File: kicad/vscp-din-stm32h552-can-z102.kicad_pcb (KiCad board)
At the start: 2 copper layers, 47.8 x 84.8 mm, 39 parts, among them J1 Conn_01x05, J2 Conn_01x02, J3 Conn_01x06, J4 Conn_01x04, J5 Conn_01x04, J6 Conn_01x03, J7 Conn_01x05, J8 Conn_01x02, J9 Conn_01x02, U1 ESP32-C3-WROOM-02-N4, U2 LM2575-3.3BT, U3 SN65HVD232, U4 R-78B3.3-1.0 (Recom)

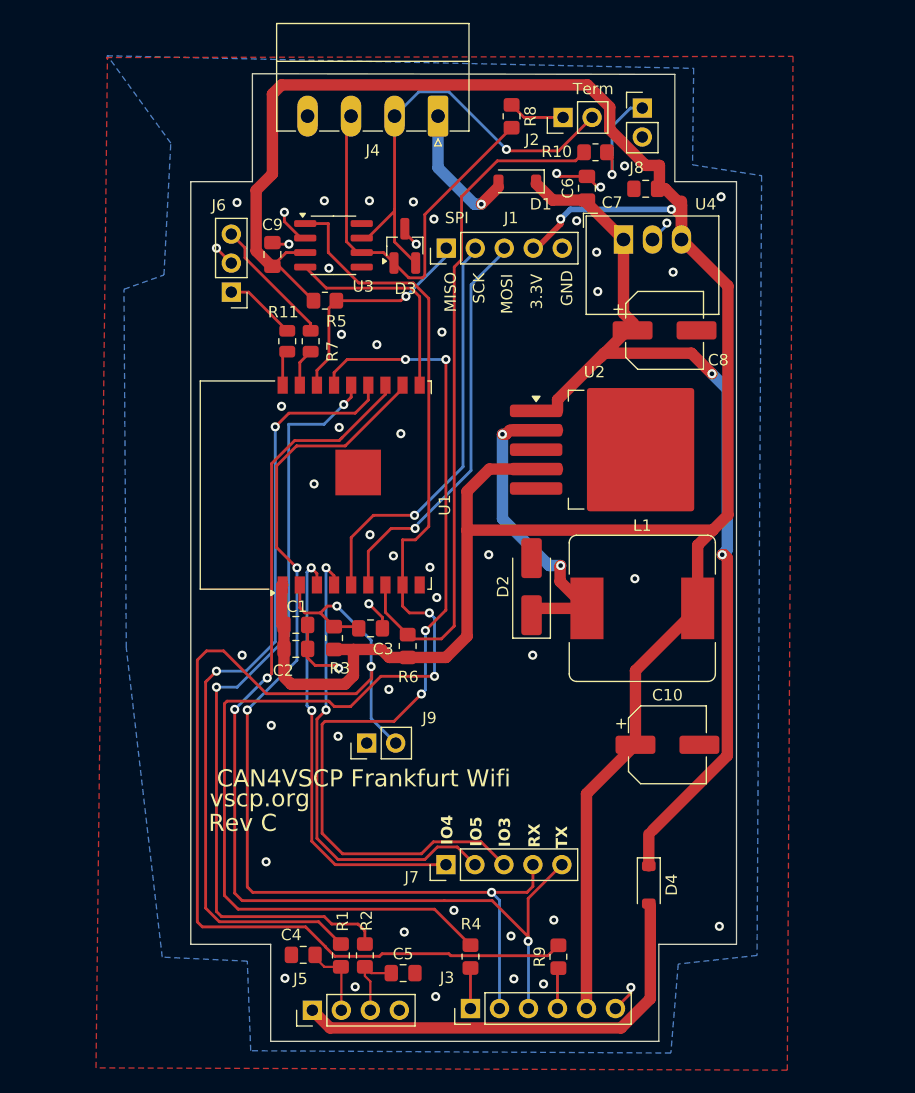
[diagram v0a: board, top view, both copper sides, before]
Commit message: Reversion A schema and PCB
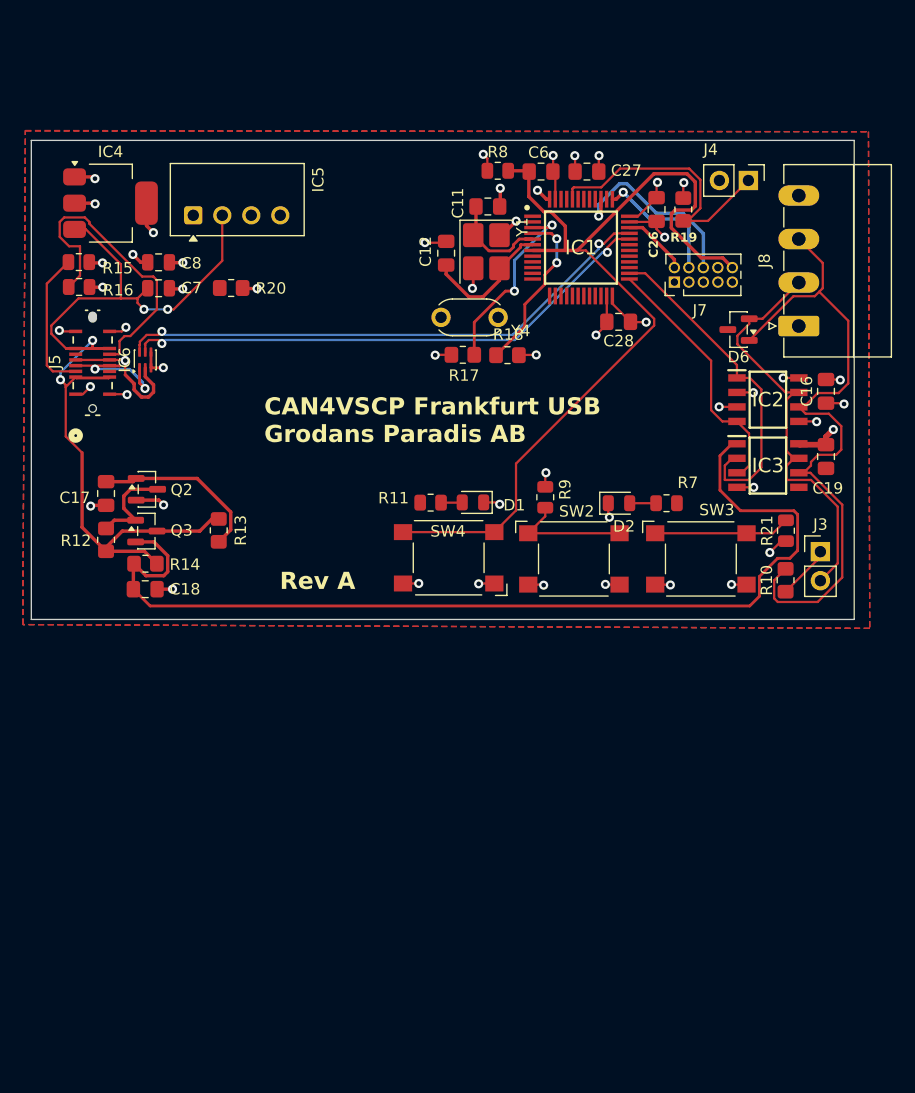
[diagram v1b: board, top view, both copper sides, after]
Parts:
- removed C1, C4, C5: 0.1uF, Capacitor_SMD:C_0805_2012Metric_Pad1.18x1.45mm_HandSolder
- removed C10: 330uF/16V, Capacitor_SMD:CP_Elec_6.3x9.9
- removed C2: 10uF, Capacitor_SMD:C_0805_2012Metric_Pad1.18x1.45mm_HandSolder
- removed C3: 1uF, Capacitor_SMD:C_0805_2012Metric_Pad1.18x1.45mm_HandSolder
- removed C9: 100nF, Capacitor_SMD:C_0805_2012Metric_Pad1.18x1.45mm_HandSolder
- removed D3: NUP2105L, Package_TO_SOT_SMD:SOT-23_Handsoldering
- removed D4: 1N5819, Diode_SMD:D_SOD-123
- removed J1: Conn_01x05, Connector_PinHeader_2.54mm:PinHeader_1x05_P2.54mm_Vertical
- removed J2, J9: Conn_01x02, Connector_PinHeader_2.54mm:PinHeader_1x02_P2.54mm_Vertical
- removed J6: Conn_01x03, Connector_PinHeader_2.54mm:PinHeader_1x03_P2.54mm_Vertical
- removed L1: SRR1240-331K, Inductor_SMD:L_Bourns_SRR1260
- removed R1, R2: 27R, Resistor_SMD:R_0805_2012Metric_Pad1.20x1.40mm_HandSolder
- removed R3, R5, R6: 10K, Resistor_SMD:R_0805_2012Metric_Pad1.20x1.40mm_HandSolder
- removed R4: 470, Resistor_SMD:R_0805_2012Metric_Pad1.20x1.40mm_HandSolder
- removed U1: ESP32-C3-WROOM-02-N4, RF_Module:ESP-WROOM-02
- removed U2: LM2575-3.3BT, Package_TO_SOT_SMD:TO-263-5_TabPin3
- removed U3: SN65HVD232, Package_SO:SOIC-8_3.9x4.9mm_P1.27mm
- removed U4: R-78B3.3-1.0 (Recom), Converter_DCDC:Converter_DCDC_RECOM_R-78B-2.0_THT
- added C11: 10p, Capacitor_SMD:C_0805_2012Metric_Pad1.18x1.45mm_HandSolder, F.Cu at (145.7, 77.6)
- added C12: 10p, Capacitor_SMD:C_0805_2012Metric_Pad1.18x1.45mm_HandSolder, F.Cu at (142.1, 81.7)
- added C16: 0.1uF, Capacitor_SMD:C_0805_2012Metric_Pad1.18x1.45mm_HandSolder, F.Cu at (175.3, 93.8)
- added C17: 22uF, Capacitor_SMD:C_0805_2012Metric_Pad1.18x1.45mm_HandSolder, F.Cu at (112.3, 102.7)
- added C18: 100nF, Capacitor_SMD:C_0805_2012Metric_Pad1.18x1.45mm_HandSolder, F.Cu at (115.7, 111.1)
- added C19: 100nF, Capacitor_SMD:C_0805_2012Metric_Pad1.18x1.45mm_HandSolder, F.Cu at (175.3, 99.5)
- added C26: 0.1uF, Capacitor_SMD:C_0805_2012Metric_Pad1.18x1.45mm_HandSolder, F.Cu at (160.5, 77.9)
- added C27: 0.1uF, Capacitor_SMD:C_0805_2012Metric_Pad1.18x1.45mm_HandSolder, F.Cu at (154.4, 74.5)
- added C28: 0.1uF, Capacitor_SMD:C_0805_2012Metric_Pad1.18x1.45mm_HandSolder, F.Cu at (157.2, 87.7)
- added D6: NUP2105L, Package_TO_SOT_SMD:SOT-23, F.Cu at (167.7, 88.4)
- added IC1: STM32C552CET6, STM32C552CET6:QFP50P900X900X160-48N, F.Cu at (153.9, 81.2)
- added IC2: TCAN3403DRQ1, TCAN3403DRQ1:SOIC127P600X175-8N, F.Cu at (170.2, 94.5)
- added IC3: ADM3050EBRIZ-RL, TCAN3403DRQ1:SOIC127P600X175-8N, F.Cu at (170.2, 100.3)
- added IC4: NCP1117-1.5_SOT223, Package_TO_SOT_SMD:SOT-223-3_TabPin2, F.Cu at (112.7, 77.3)
- added IC5: TME-0505S, Converter_DCDC:Converter_DCDC_TRACO_TME_03xxS_05xxS_12xxS_Single_THT, F.Cu at (119.9, 78.4)
- added IC6: ECMF02-2AMX6, Package_DFN_QFN:ST_UQFN-6L_1.5x1.7mm_P0.5mm, F.Cu at (115.7, 91.0)
- added Q2: 2N7002, Package_TO_SOT_SMD:SOT-23, F.Cu at (115.9, 102.4)
- added Q3: 2N7002, Package_TO_SOT_SMD:SOT-23, F.Cu at (115.8, 106.0)
- added R12: 10K, Resistor_SMD:R_0805_2012Metric_Pad1.20x1.40mm_HandSolder, F.Cu at (112.3, 106.8)
- added R13: 100K, Resistor_SMD:R_0805_2012Metric_Pad1.20x1.40mm_HandSolder, F.Cu at (122.2, 106.0)
- added R14: 0R, Resistor_SMD:R_0805_2012Metric_Pad1.20x1.40mm_HandSolder, F.Cu at (115.7, 108.9)
- added R15: 5k1_0603_100mW_1%_E24_Chip-Resistor, Resistor_SMD:R_0805_2012Metric, F.Cu at (109.9, 82.5)
- added R16: 5k1_0603_100mW_1%_E24_Chip-Resistor, Resistor_SMD:R_0805_2012Metric, F.Cu at (109.9, 84.7)
- added R17: 0K, Resistor_SMD:R_0805_2012Metric_Pad1.20x1.40mm_HandSolder, F.Cu at (143.5, 90.6)
- added R18: 0K, Resistor_SMD:R_0805_2012Metric_Pad1.20x1.40mm_HandSolder, F.Cu at (147.4, 90.6)
- added R19: 10K, Resistor_SMD:R_0805_2012Metric_Pad1.20x1.40mm_HandSolder, F.Cu at (162.8, 77.9)
- added R20: 0R, Resistor_SMD:R_0805_2012Metric_Pad1.20x1.40mm_HandSolder, F.Cu at (123.2, 84.7)
- added R21: 10K, Resistor_SMD:R_0805_2012Metric, F.Cu at (171.8, 106.0)
- added SW2: Control 1, Button_Switch_SMD:SW_SPST_Omron_B3FS-100xP, F.Cu at (153.3, 108.5)
- added SW3: Control 2, Button_Switch_SMD:SW_SPST_Omron_B3FS-100xP, F.Cu at (164.4, 108.5)
- added SW4: RESET, Button_Switch_SMD:SW_SPST_Omron_B3FS-100xP, F.Cu at (142.3, 108.4)
- added Y1: Crystal_GND24, Crystal:Crystal_SMD_TXC_7M-4Pin_3.2x2.5mm_HandSoldering, F.Cu at (145.6, 81.6)
- added Y4: 32.768kHz, Crystal:Resonator-2Pin_W6.0mm_H3.0mm, F.Cu at (141.6, 87.3)
- C6: value 10uF -> 1uF
- C7: value 1uF -> 10u_0805_X7R_10%_10V_-40C..125C_Chip-Capacitor; footprint Capacitor_SMD:C_0805_2012Metric_Pad1.18x1.45mm_HandSolder -> Capacitor_SMD:C_0805_2012Metric
- C8: value 100uF/50V -> 10u_0805_X7R_10%_10V_-40C..125C_Chip-Capacitor; footprint Capacitor_SMD:CP_Elec_6.3x9.9 -> Capacitor_SMD:C_0805_2012Metric
- D1: value 1N5819 -> LED (Green); footprint Diode_SMD:D_SOD-123 -> LED_SMD:LED_0805_2012Metric
- D2: value 1N5822 -> LED (Blue); footprint Diode_SMD:D_SMA_Handsoldering -> LED_SMD:LED_0805_2012Metric
- J3: value Conn_01x06 -> Conn_01x02; footprint Connector_PinHeader_2.54mm:PinHeader_1x06_P2.54mm_Vertical -> Connector_PinHeader_2.54mm:PinHeader_1x02_P2.54mm_Vertical
- J4: value Conn_01x04 -> Conn_01x02; footprint Connector_Phoenix_MC:PhoenixContact_MC_1,5_4-G-3.81_1x04_P3.81mm_Horizontal -> Connector_PinHeader_2.54mm:PinHeader_1x02_P2.54mm_Vertical
- J5: value Conn_01x04 -> USB4145-03-0230-C; footprint Connector_PinHeader_2.54mm:PinHeader_1x04_P2.54mm_Vertical -> USB4145-03-0230-C:CONN_USB4145-03-0230-C_GCT
- J7: value Conn_01x05 -> Conn_ARM_JTAG_SWD_10; footprint Connector_PinHeader_2.54mm:PinHeader_1x05_P2.54mm_Vertical -> Connector_PinHeader_1.27mm:PinHeader_2x05_P1.27mm_Vertical
- J8: value Conn_01x02 -> Conn_01x04; footprint Connector_PinHeader_2.54mm:PinHeader_1x02_P2.54mm_Vertical -> Connector_Phoenix_MC:PhoenixContact_MC_1,5_4-G-3.81_1x04_P3.81mm_Horizontal
- R10: value 330R -> 120R
- R8: value 120R -> 10K; footprint Resistor_SMD:R_0805_2012Metric_Pad1.20x1.40mm_HandSolder -> Resistor_SMD:R_0805_2012Metric
- R9: value 470 -> 10K; footprint Resistor_SMD:R_0805_2012Metric_Pad1.20x1.40mm_HandSolder -> Resistor_SMD:R_0805_2012Metric
- moved J5 59.9 mm to (111.1, 91.3)
- moved J7 54.8 mm to (162.1, 84.2)
- moved J3 50.4 mm to (174.8, 107.8), turned to 0 degrees
- moved C8 44.7 mm to (116.9, 82.5)
- moved C7 43.5 mm to (116.9, 84.8), turned to 0 degrees
- moved R10 41.0 mm to (171.8, 110.3), turned to 90 degrees
- moved R9 40.3 mm to (150.8, 103.1), turned to -90 degrees
- moved R7 34.2 mm to (161.4, 103.6), turned to 0 degrees
- moved D1 28.4 mm to (144.4, 103.5)
- moved J4 27.8 mm to (168.5, 75.3), turned to -90 degrees
- moved J8 23.5 mm to (173.0, 88.1), turned to 90 degrees
- moved R11 18.9 mm to (140.7, 103.5), turned to 0 degrees
- moved D2 10.6 mm to (157.2, 103.6), turned to 0 degrees
- moved R8 4.92 mm to (146.6, 74.5), turned to 0 degrees
- moved C6 4.28 mm to (150.4, 74.5), turned to 0 degrees
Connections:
- C6 pad 1: +28V -> /MCU/NRST
- C7 pad 1: +3V3 -> +5V
- C8 pad 1: +28V -> +3.3V
- D1 pad 1: +28V -> GND
- D2 pad 1: Net-(D2-K) -> GND
- D2 pad 2: GND -> Net-(D2-A)
- J3 pad 2: /rx -> /CAN/CANH
- J4 pad 1: Net-(D1-A) -> /MCU/BOOT0
- J4 pad 2: Net-(J2-Pin_2) -> GND
- J7 pad 1: /io4 -> +3.3V
- J7 pad 2: /io5 -> /MCU/SWDIO
- J7 pad 3: /io3 -> GND
- J7 pad 4: /rx -> /MCU/SWCLK
- J7 pad 5: /tx -> GND
- J8 pad 1: Net-(J8-Pin_1) -> unconnected-(J8-Pin_1-Pad1)
- J8 pad 2: GND -> /CAN/CANH
- R10 pad 1: Net-(J8-Pin_1) -> Net-(J3-Pin_1)
- R10 pad 2: /boff -> /CAN/CANL
- R11 pad 1: /leda -> leda
- R11 pad 2: Net-(J6-Pin_1) -> Net-(D1-A)
- R7 pad 1: Net-(J6-Pin_3) -> Net-(D2-A)
- R7 pad 2: /ledb -> ledb
- R8 pad 1: Net-(J2-Pin_1) -> +3.3V
- R8 pad 2: Net-(J4-Pin_3) -> /MCU/NRST
- R9 pad 1: Net-(J3-Pin_4) -> +3.3V
- R9 pad 2: /reset -> CTRL1
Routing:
- net +3V3: track 237.4 -> 0.00 mm, vias 2 -> 0
- net /txcan: track 111.8 -> 0.00 mm, vias 2 -> 0
- net /reset: track 98.9 -> 0.00 mm, vias 2 -> 0
- net /tx: track 93.8 -> 0.00 mm, vias 3 -> 0
- net /rx: track 91.3 -> 0.00 mm, vias 3 -> 0
- net +5VD: track 0.00 -> 88.1 mm
- net +28V: track 85.3 -> 0.00 mm, vias 2 -> 0
- net +5V: track 0.00 -> 84.5 mm, vias 0 -> 4
- net /MCU/NRST: track 0.00 -> 82.0 mm
- net /io3: track 78.9 -> 0.00 mm, vias 4 -> 0
- net Net-(U1-IO18): track 69.8 -> 0.00 mm, vias 2 -> 0
- net Net-(U1-IO19): track 68.7 -> 0.00 mm, vias 2 -> 0
- net /CAN/CANL: track 0.00 -> 60.3 mm
- net /boff: track 60.1 -> 0.00 mm
- net USB_DP: track 0.00 -> 48.2 mm, vias 0 -> 2
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- added copper zone on In2.Cu, net +3.3V
- added copper zone on B.Cu, net +5VP
- added copper zone on In1.Cu, net GND
- added copper zone on F.Cu, net GNDD
- removed copper zone on B.Cu, net GND
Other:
- board size 47.8 x 84.8 mm -> 72.1 x 42 mm
- copper layers 2 -> 4
- board text added: "CAN4VSCP Frankfurt USB Grodans Paradis AB"
- board text added: "Rev A"
- board text removed: "+3.3V"
- board text removed: "3.3V"
- board text removed: "CAN4VSCP Frankfurt Wifi"
- board text removed: "CANH"
- board text removed: "CANL"
- board text removed: "D+"
- board text removed: "D-"
- board text removed: "FLASH"
- board text removed: "GND"
- board text removed: "IO3"
- board text removed: "IO4"
- board text removed: "IO5"
- board text removed: "MISO"
- board text removed: "MOSI"
- board text removed: "PWR"
- board text removed: "RX"
- board text removed: "Reset"
- board text removed: "Rev C"
- board text removed: "SCK"
- board text removed: "SPI"
- board text removed: "TX"
- board text removed: "Term"
- board text removed: "vscp.org"
- board text removed: "www.grodansparadis.com"
